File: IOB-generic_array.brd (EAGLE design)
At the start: 104.1 x 106.7 mm, 33 parts

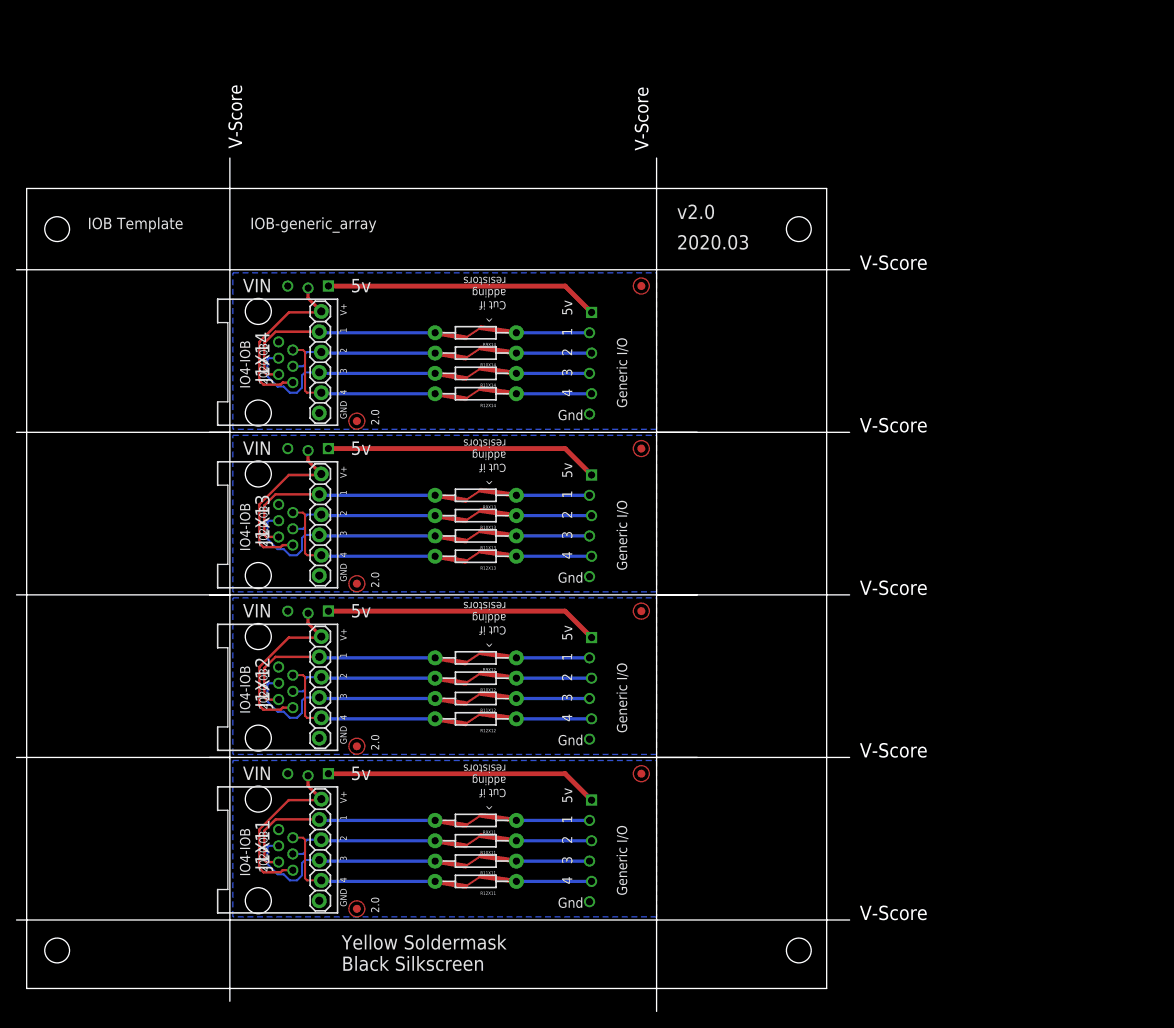
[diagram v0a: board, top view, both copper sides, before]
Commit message: added array...
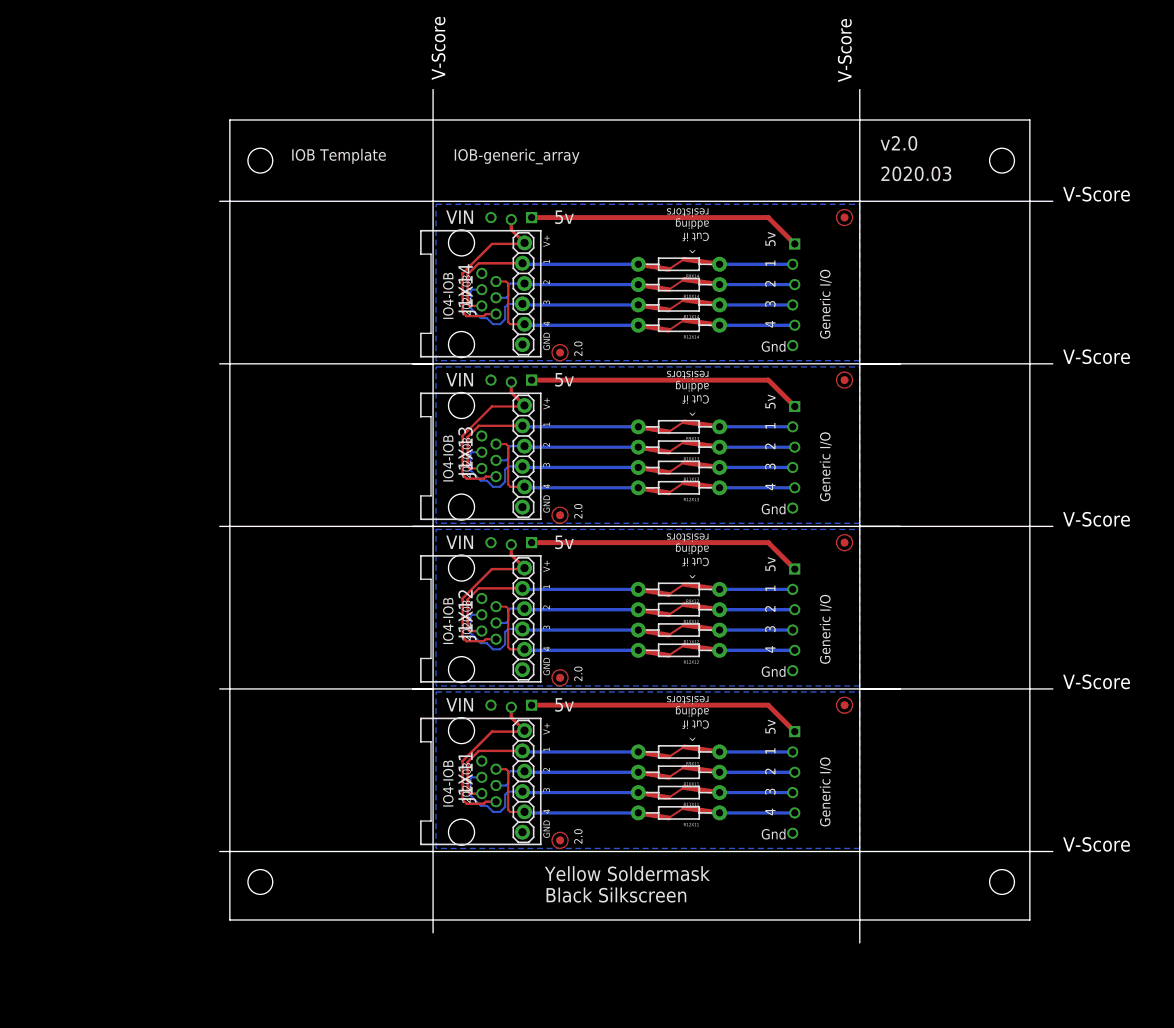
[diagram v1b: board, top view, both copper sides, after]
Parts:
- moved R12X1 26.9 mm to (0.00, 0.00)
- moved FID1X11 26.8 mm to (41.3, 9.96)
- moved FID1X12 26.8 mm to (41.3, 30.3)
- moved FID1X13 26.8 mm to (41.3, 50.6)
- moved FID1X14 26.8 mm to (41.3, 70.9)
- moved IOBX11 26.8 mm to (25.4, 8.56)
- moved IOBX12 26.8 mm to (25.4, 28.9)
- moved IOBX13 26.8 mm to (25.4, 49.2)
- moved J1X11 26.8 mm to (32.8, 17.3)
- moved J1X12 26.8 mm to (32.8, 37.6)
- moved J1X13 26.8 mm to (32.8, 58.0)
- moved J1X14 26.8 mm to (32.8, 78.3)
- moved R10X11 26.8 mm to (56.1, 18.5)
- moved R10X12 26.8 mm to (56.1, 38.8)
- moved R10X13 26.8 mm to (56.1, 59.1)
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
